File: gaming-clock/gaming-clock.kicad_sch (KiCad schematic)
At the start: 10 parts, among them J1 USB_C_Receptacle_USB2.0, U1 ESP32-C3-WROOM-02, U2 LM1117GS-3.3

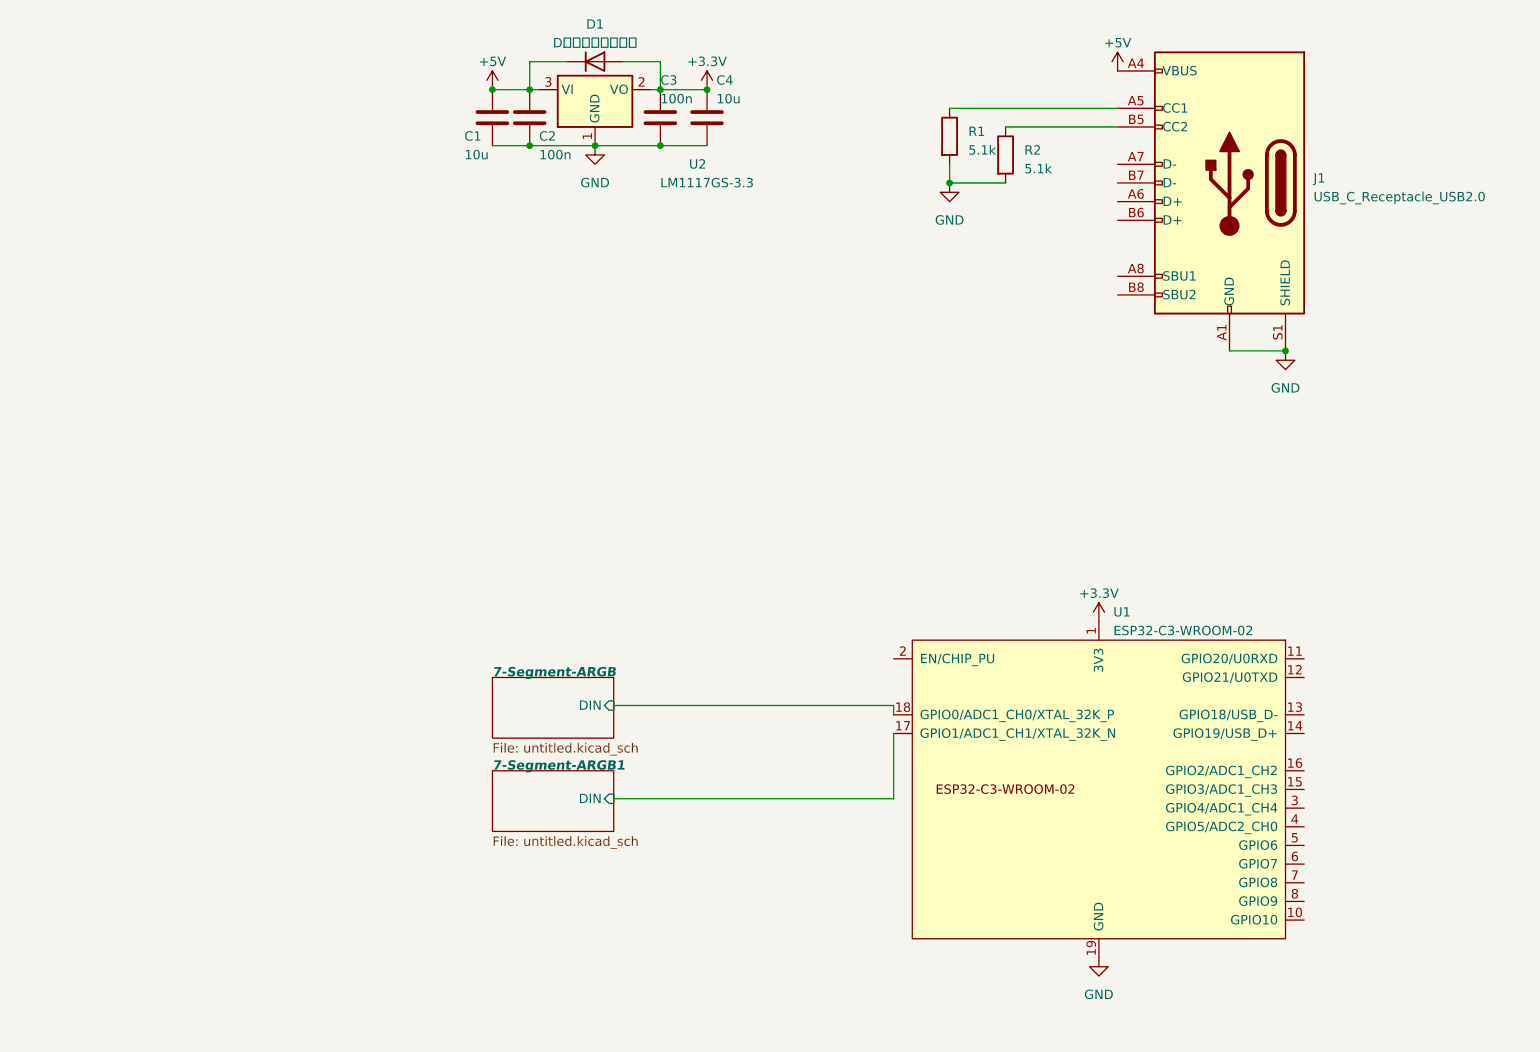
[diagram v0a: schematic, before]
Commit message: c
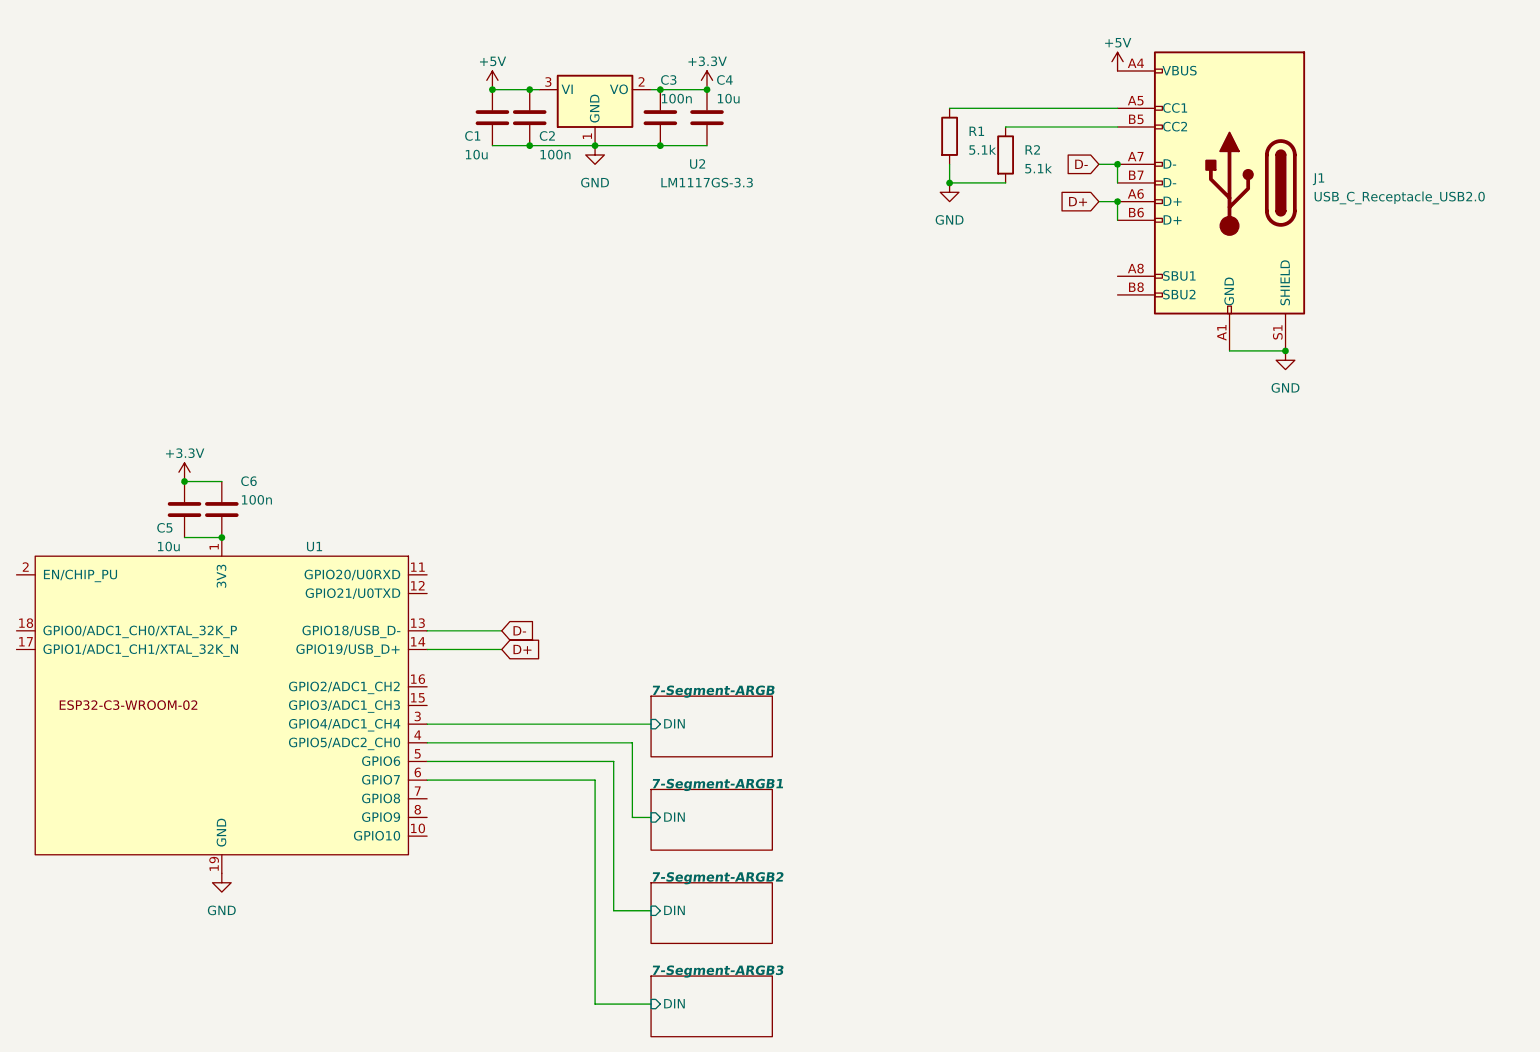
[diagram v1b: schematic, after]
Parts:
- removed D1: DＧＳ１０１０ＦＬ, Diode_SMD:D_SOD-123F, symbol Device:D
- added C5: 10u, Capacitor_SMD:C_0603_1608Metric_Pad1.08x0.95mm_HandSolder, symbol Device:C
- added C6: 100n, Capacitor_SMD:C_0603_1608Metric_Pad1.08x0.95mm_HandSolder, symbol Device:C
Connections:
- net +3.3V: now also C5.1, C6.1; no longer U1.1 (3V3)
- net 7-Segment-ARGB/DIN: now also U1.3 (GPIO4/ADC1_CH4); no longer U1.18 (GPIO0/ADC1_CH0/XTAL_32K_P)
- net 7-Segment-ARGB1/DIN: now also U1.4 (GPIO5/ADC2_CH0); no longer U1.17 (GPIO1/ADC1_CH1/XTAL_32K_N)
- net D-: now reaches U1.13 (GPIO18/USB_D-)
- net D-: now also J1.A7 (D-), J1.B7 (D-)
- net D+: now reaches U1.14 (GPIO19/USB_D+)
- net D+: now also J1.A6 (D+), J1.B6 (D+)
- net 7-Segment-ARGB2/DIN: now reaches U1.5 (GPIO6)
- net 7-Segment-ARGB3/DIN: now reaches U1.6 (GPIO7)
- new net: C5.2, C6.2, U1.1 (3V3)
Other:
- added sheet 7-Segment-ARGB2 (untitled.kicad_sch)
- added sheet 7-Segment-ARGB3 (untitled.kicad_sch)
- moved on the sheet: U1
